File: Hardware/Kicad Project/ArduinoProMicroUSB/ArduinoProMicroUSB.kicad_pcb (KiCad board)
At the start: 4 copper layers, 31.1 x 26 mm, 51 parts, among them J3 Display FPC, Q1 MMBT3904, U1 RV-3028-C7, U3 USB-AB, U5 ATMEGA32U4QFN, Y1 16MHz

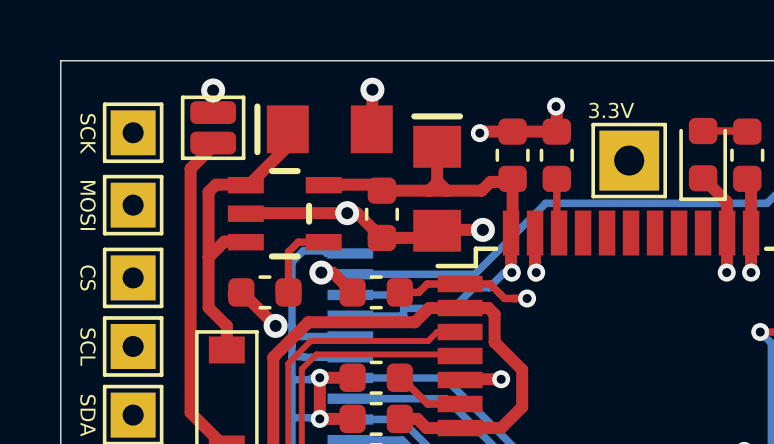
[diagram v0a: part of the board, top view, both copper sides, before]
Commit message: gif
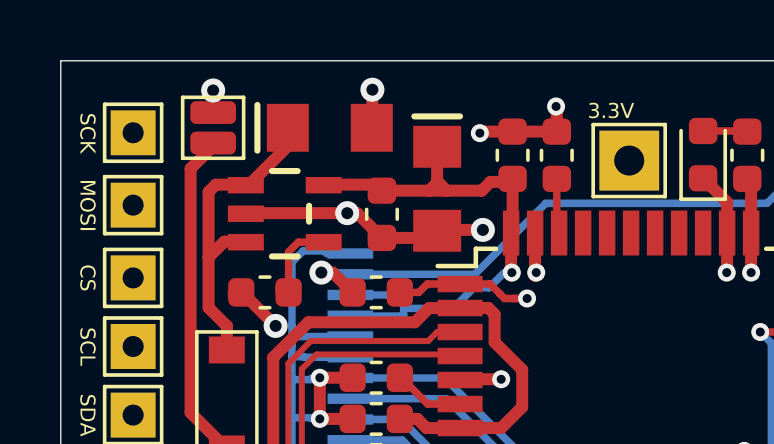
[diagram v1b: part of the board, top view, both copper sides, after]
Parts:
- moved C1 0.05 mm to (135.5, 76.7)
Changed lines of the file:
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@@
   )
   (module Capacitors:EIA3216 (layer F.Cu)
-    (at 135.46074 76.708 180)
+    (at 135.46074 76.6572 180)
     (descr "GENERIC EIA 3216 (1206) POLARIZED TANTALUM CAPACITOR")
     (tags "GENERIC EIA 3216 (1206) POLARIZED TANTALUM CAPACITOR")

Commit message: rev 0.2
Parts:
- renumbered UE to U2
